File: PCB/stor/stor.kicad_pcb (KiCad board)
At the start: 4 copper layers, 21 x 55.7 mm, 45 parts, among them J1 Conn_01x04_Socket, SW1 TS1603-TZ38HBM, SW2 TS1603-TZ38HBM, U1 STM32H723VGT6, U2 TYPE-C 24P-GTJB 040, U3 USB3300-EZK-TR, U4 TPS62177DQCR, X1 25mhz, X2 32.768k, X3 24mhz

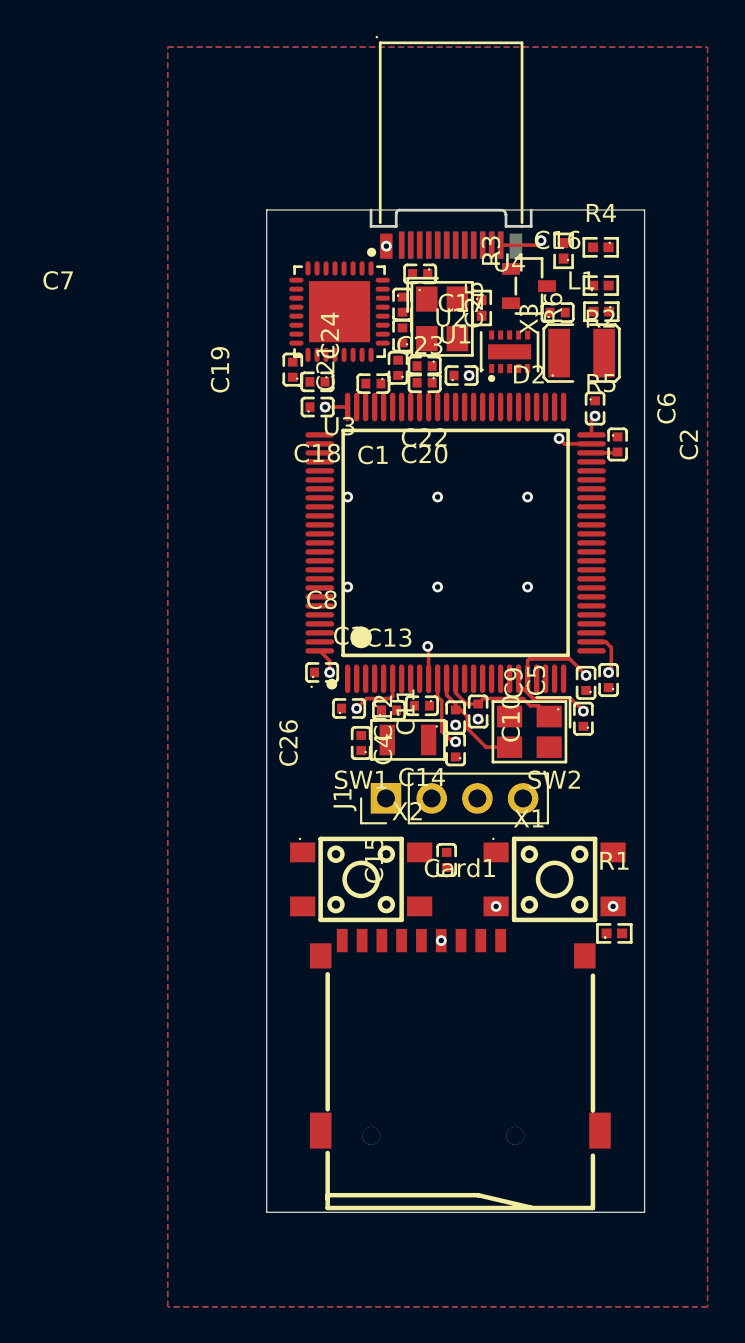
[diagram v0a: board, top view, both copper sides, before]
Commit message: soo much routing
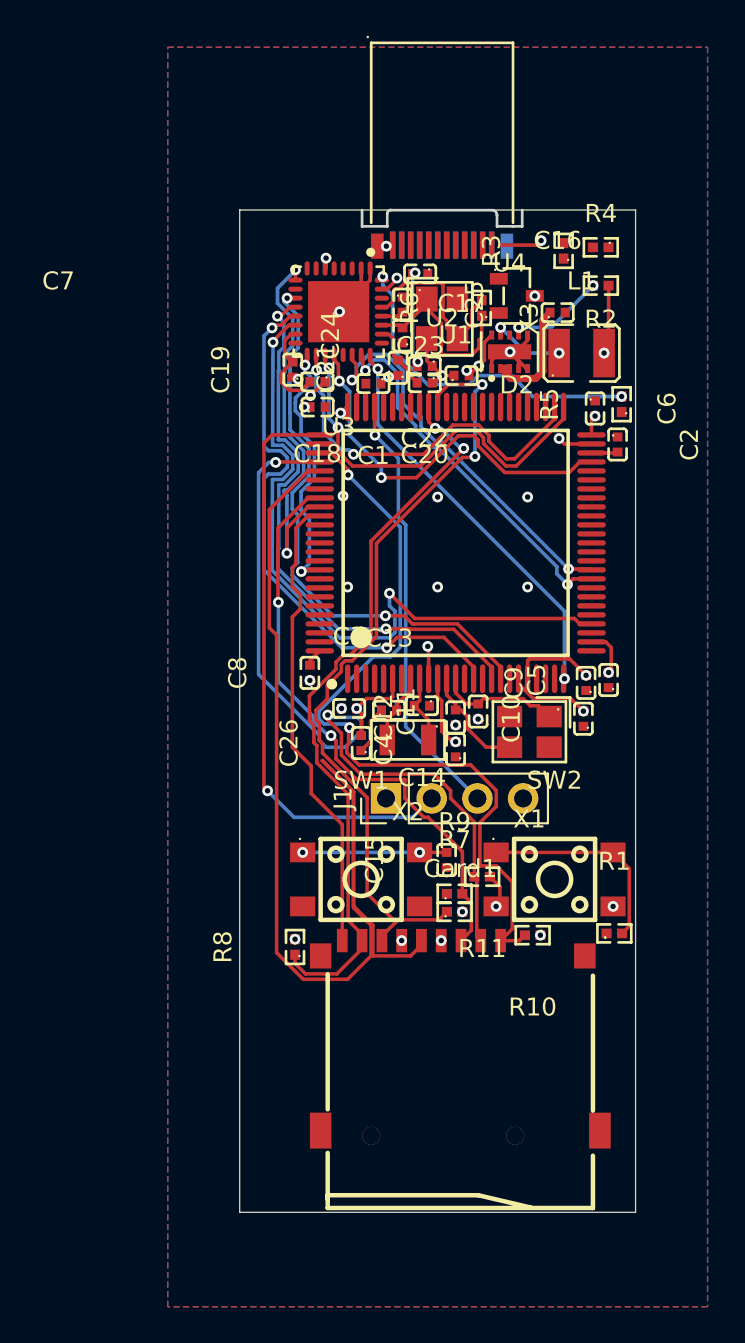
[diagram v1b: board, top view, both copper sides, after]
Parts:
- added R10: 10k, easyeda2kicad:R0402, F.Cu at (125.3, 79.3)
- added R11: 10k, easyeda2kicad:R0402, F.Cu at (122.5, 76.1)
- added R7: 10k, easyeda2kicad:R0402, F.Cu at (120.9, 78.0)
- added R8: 10k, easyeda2kicad:R0402, F.Cu at (112.1, 80.0)
- added R9: 10k, easyeda2kicad:R0402, F.Cu at (120.9, 77.0)
- moved R5 5.27 mm to (130.2, 49.8), turned to 90 degrees
- moved D2 0.87 mm to (124.4, 43.8)
- moved C8 0.68 mm to (112.9, 64.8), turned to 90 degrees
- moved U2 0.50 mm to (120.2, 41.0)
- turned R6 to 90 degrees
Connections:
- U1 pad 80: unconnected-(U1-PC12-Pad80) -> /PC12
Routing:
- net /PC12: track 0.00 -> 61.2 mm
- net /PC11: track 0.00 -> 43.6 mm, vias 0 -> 2
- net /PC10: track 0.00 -> 43.1 mm, vias 0 -> 2
- net /PC8: track 0.00 -> 43.0 mm, vias 0 -> 2
- net /PC9: track 0.00 -> 40.5 mm, vias 0 -> 2
- net /PA5: track 0.00 -> 38.0 mm, vias 0 -> 2
- net /SWCLK: track 0.00 -> 32.9 mm, vias 0 -> 1
- net /PD2: track 0.00 -> 31.8 mm, vias 0 -> 2
- net /PC3: track 0.00 -> 31.2 mm, vias 0 -> 2
- net /PC0: track 0.00 -> 31.1 mm, vias 0 -> 2
- net /PC2: track 0.00 -> 31.0 mm, vias 0 -> 2
- net /PD4: track 0.00 -> 25.5 mm
- net /SWDIO: track 0.00 -> 24.1 mm, vias 0 -> 1
- net /PA3: track 0.00 -> 22.5 mm, vias 0 -> 2
- net /PB1: track 0.00 -> 21.8 mm, vias 0 -> 2
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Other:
- board size 21 x 55.7 mm -> 22 x 55.7 mm
